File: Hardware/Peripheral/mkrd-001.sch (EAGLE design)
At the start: 5 parts

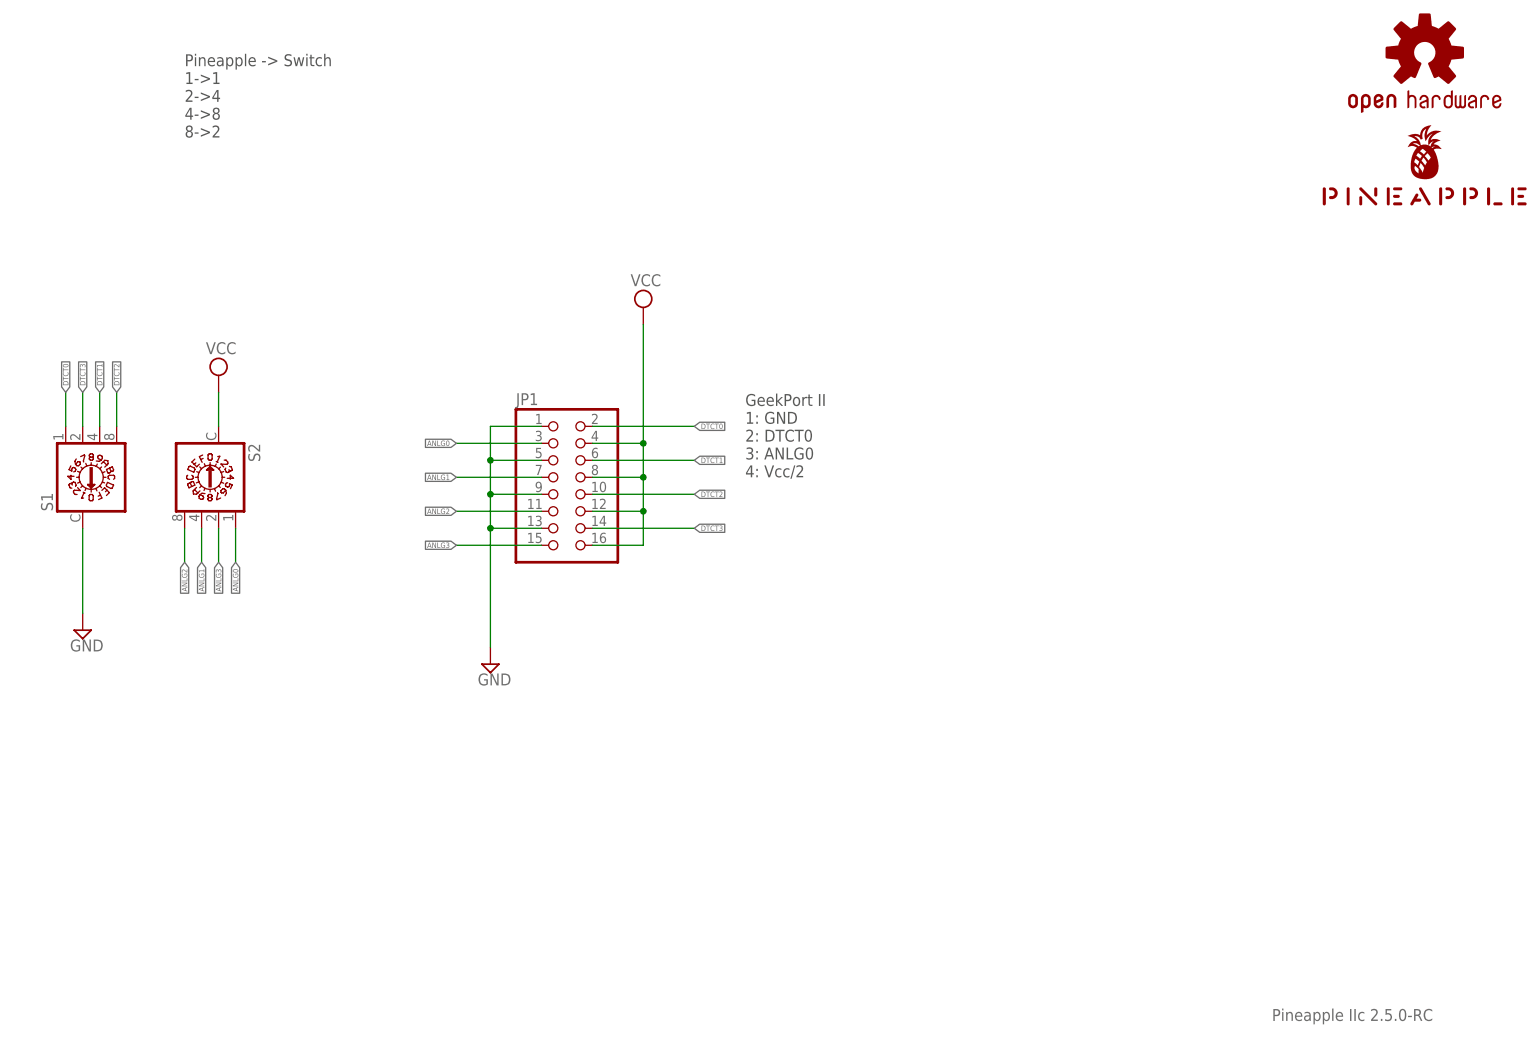
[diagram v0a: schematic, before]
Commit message: First try.
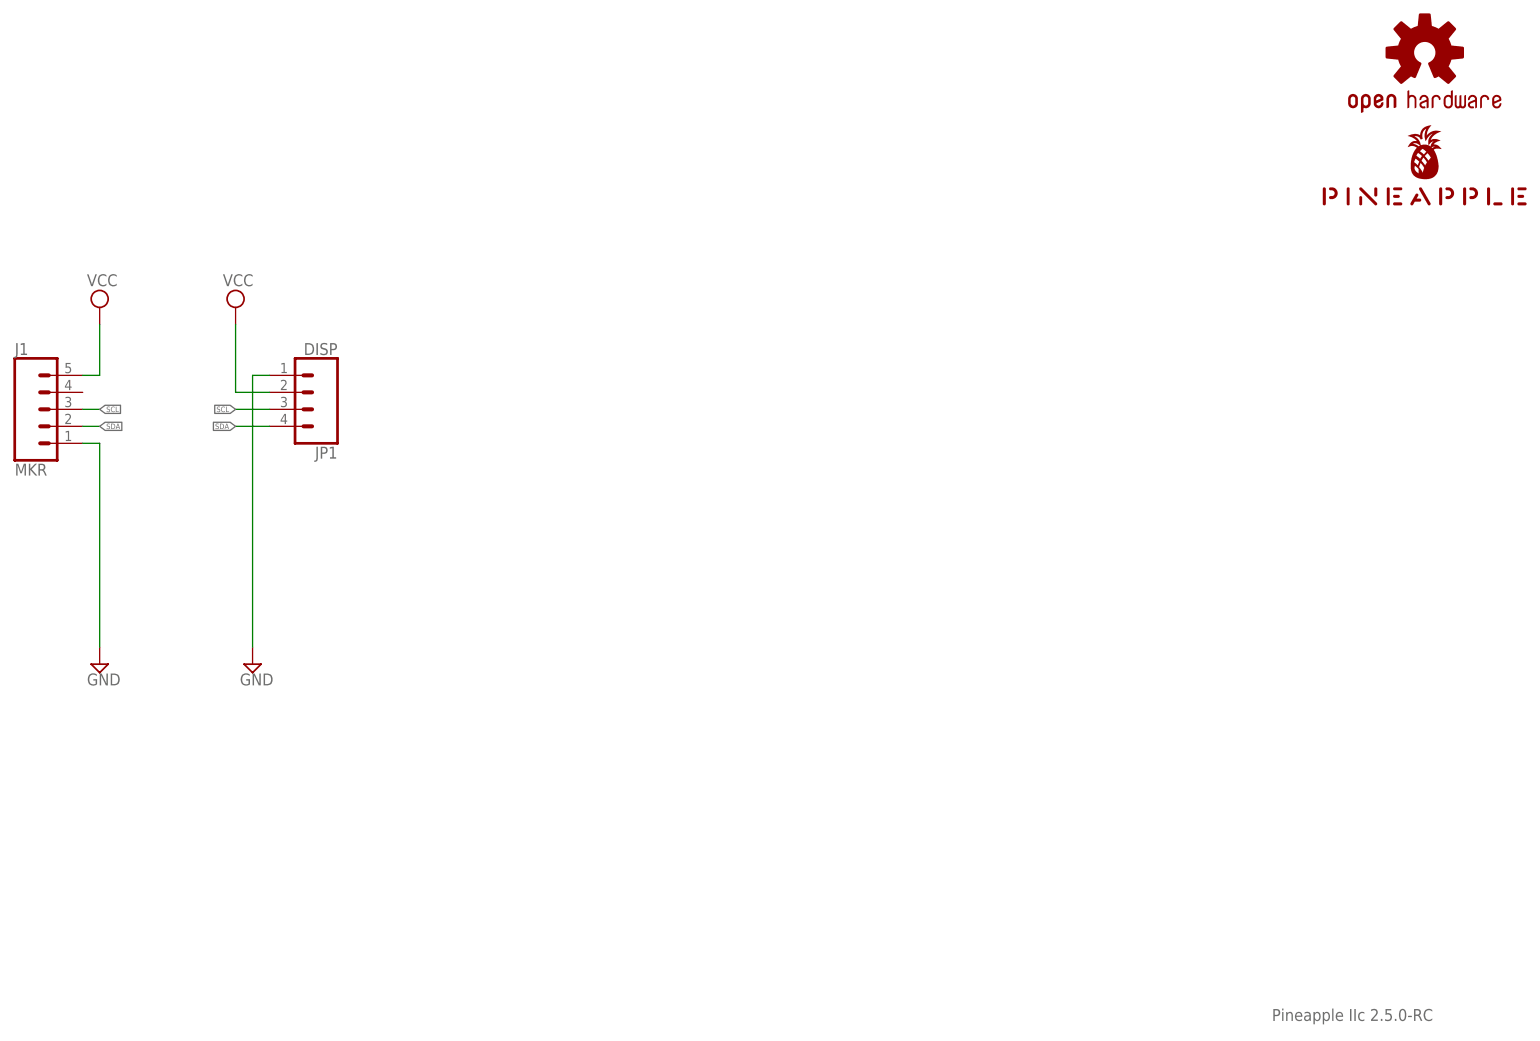
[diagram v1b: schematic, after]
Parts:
- removed S1, S2: (no value), switch-dil:A1353HEX
- added J1: MKR, SparkFun-Connectors:CONN_05JST
- JP1: value (none) -> DISP; device pinhead:PINHD-2X8 -> SparkFun-Connectors:CONN_04
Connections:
- removed net ANLG0: JP1.3, S2.1
- removed net ANLG1: JP1.7, S2.4
- removed net ANLG2: JP1.11, S2.8
- removed net ANLG3: JP1.15, S2.2
- removed net DTCT0: JP1.2, S1.1
- removed net DTCT1: JP1.6, S1.4
- removed net DTCT2: JP1.10, S1.8
- removed net DTCT3: JP1.14, S1.2
- new net SCL: J1.3, JP1.3
- new net SDA: J1.2, JP1.4
- net GND: now also J1.1; no longer JP1.13, JP1.5, JP1.9, S1.C
- net VCC: now also J1.5, JP1.2; no longer JP1.12, JP1.16, JP1.4, JP1.8, S2.C
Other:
- note removed: "GeekPort II 1: GND 2: DTCT0 3: ANLG0 4: Vcc/2"
- note removed: "Pineapple -> Switch 1->1 2->4 4->8 8->2"
